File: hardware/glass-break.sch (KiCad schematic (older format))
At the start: 33 parts, among them P1 USB_OTG, SW1 SW_PUSH, SW2 SW_PUSH, SW3 SW_PUSH, U1 esp12, U11 SPX3819, U2 OP275, U3 electret_microphone

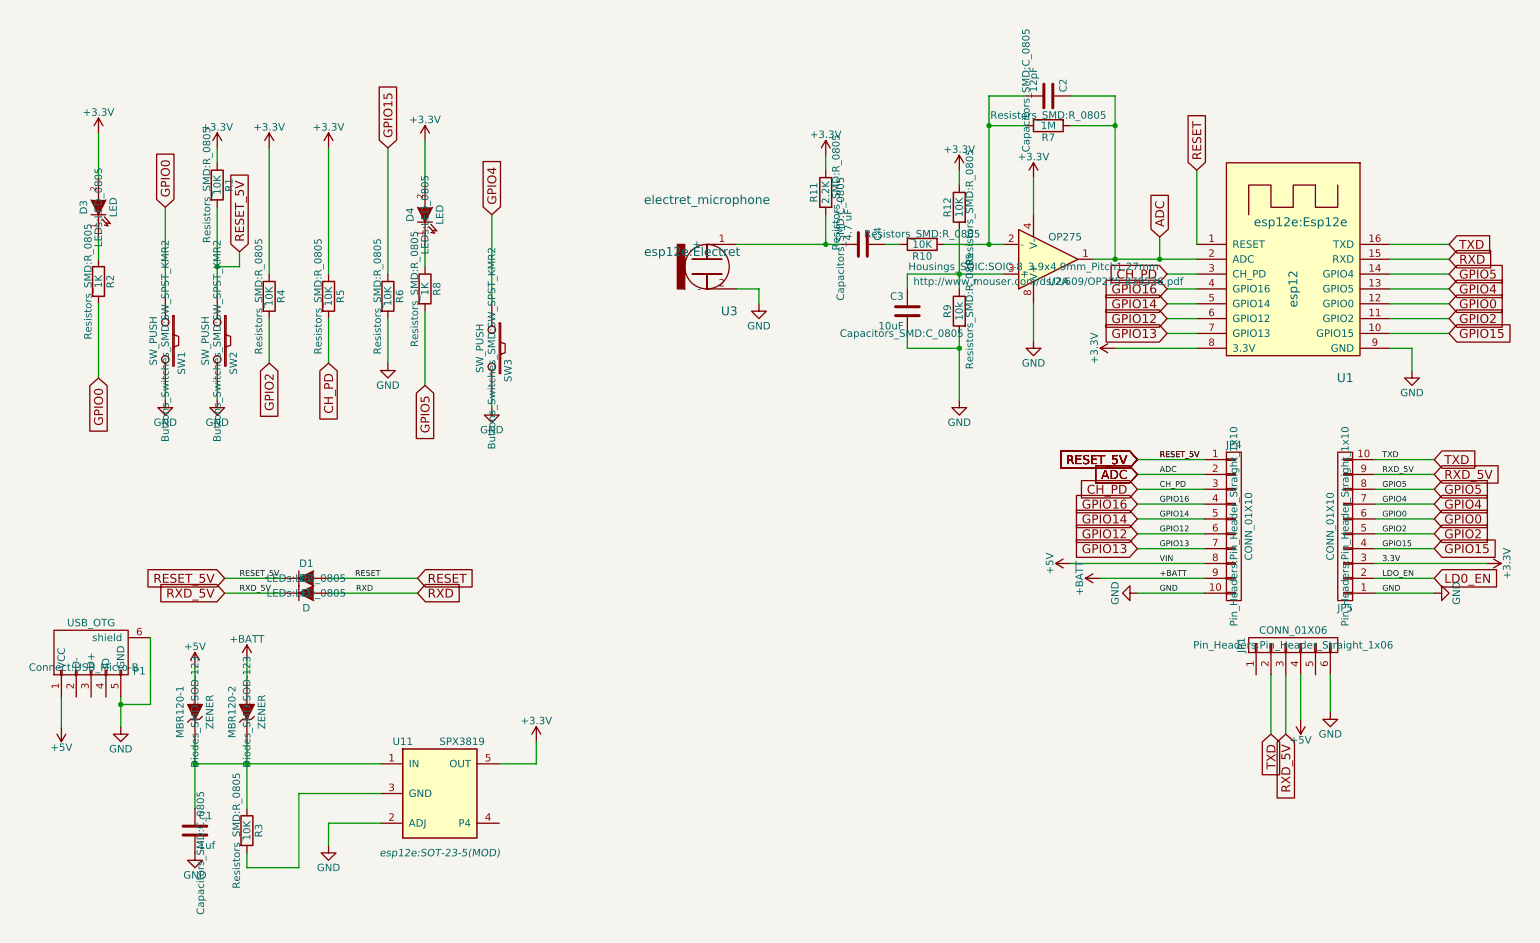
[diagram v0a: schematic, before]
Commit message: update
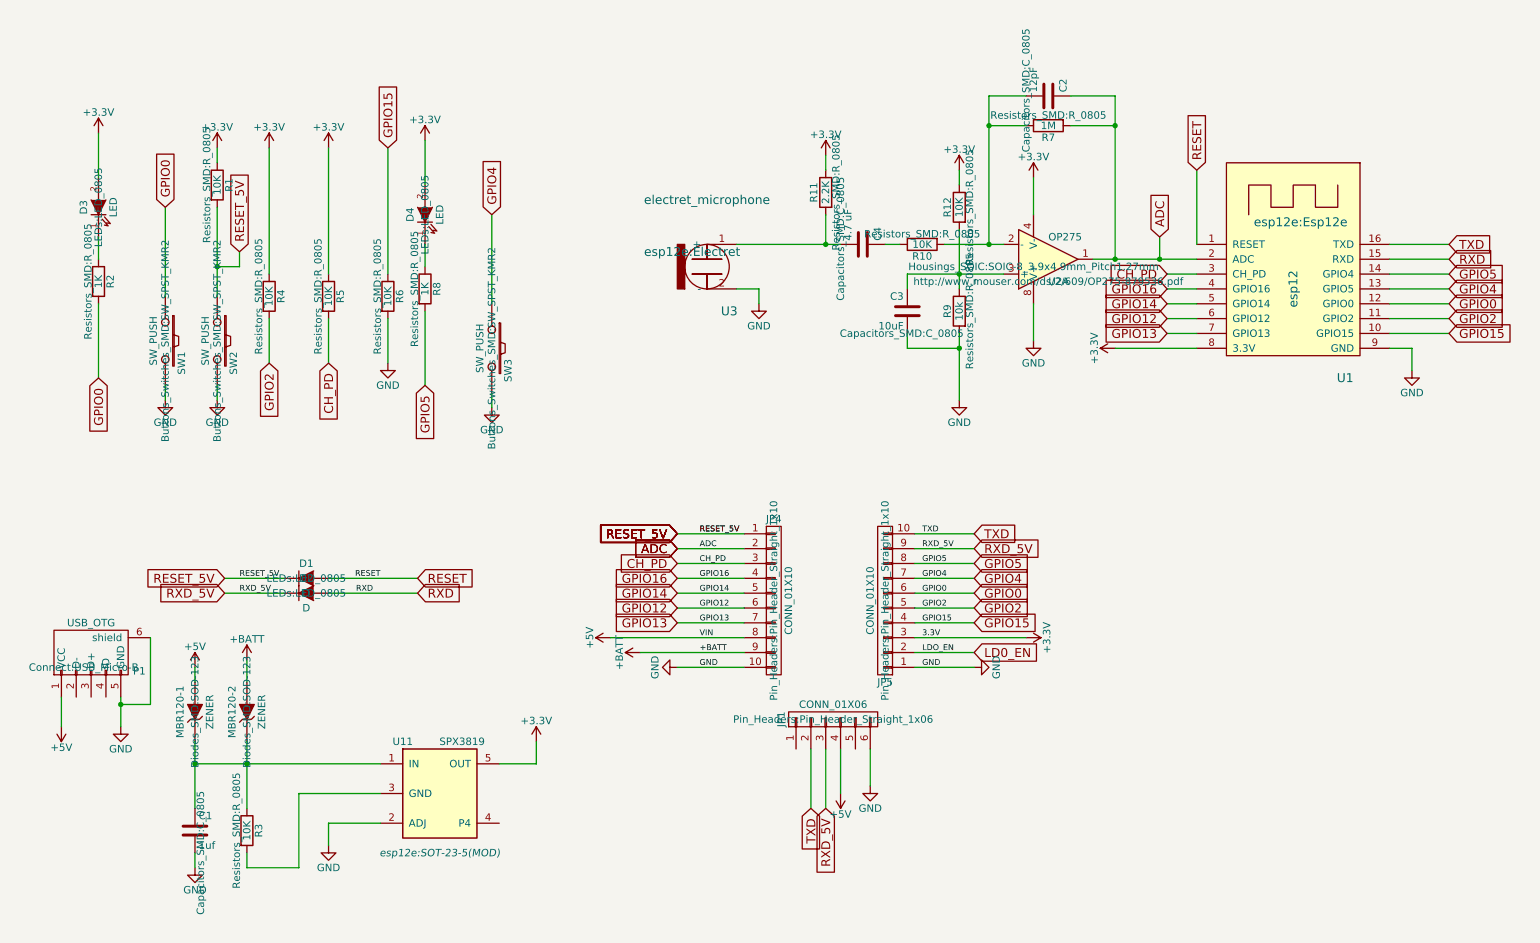
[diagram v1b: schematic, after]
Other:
- moved on the sheet: JP1, JP4, JP5
